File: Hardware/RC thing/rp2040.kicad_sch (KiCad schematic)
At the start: 29 parts, among them J2 2171790001, SW5 TL3342F160QG_TR, SW8 TL3342F160QG_TR, U2 RP2040, U3 W25Q128JVS, Y3 Crystal_GND24_Small

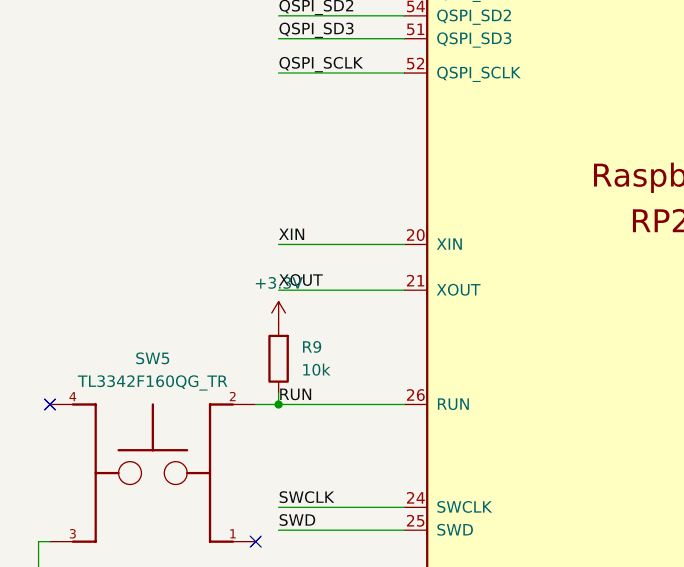
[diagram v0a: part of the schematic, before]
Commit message: G will be touched tonight
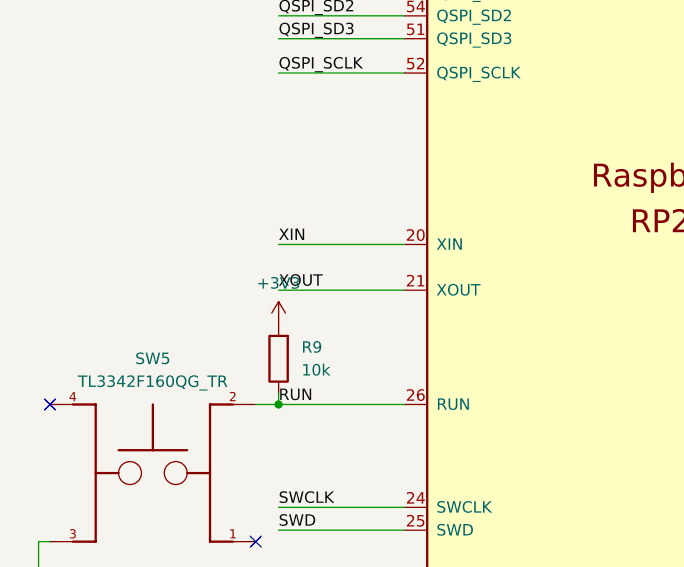
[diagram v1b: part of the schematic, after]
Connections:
- net +3.3V is gone; now on net +3V3: R9.2
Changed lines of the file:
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@@
 			)
 		)
-		(property "Value" "+3.3V"
+		(property "Value" "+3V3"
 			(at 158.75 131.318 0)
 			(effects
